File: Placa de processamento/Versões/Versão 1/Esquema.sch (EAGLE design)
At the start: 17 parts, among them IC1 5V, IC2 5V

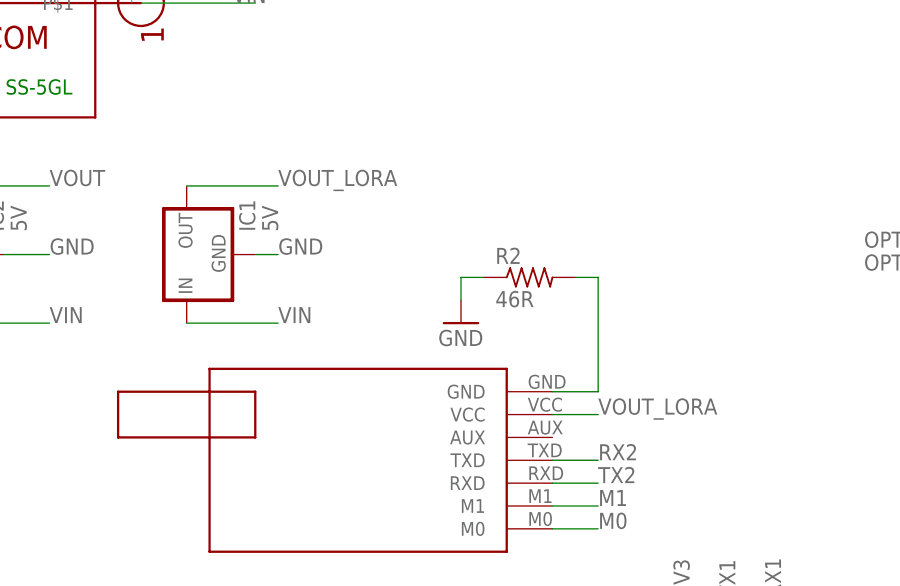
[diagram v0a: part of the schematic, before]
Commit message: uptate boards
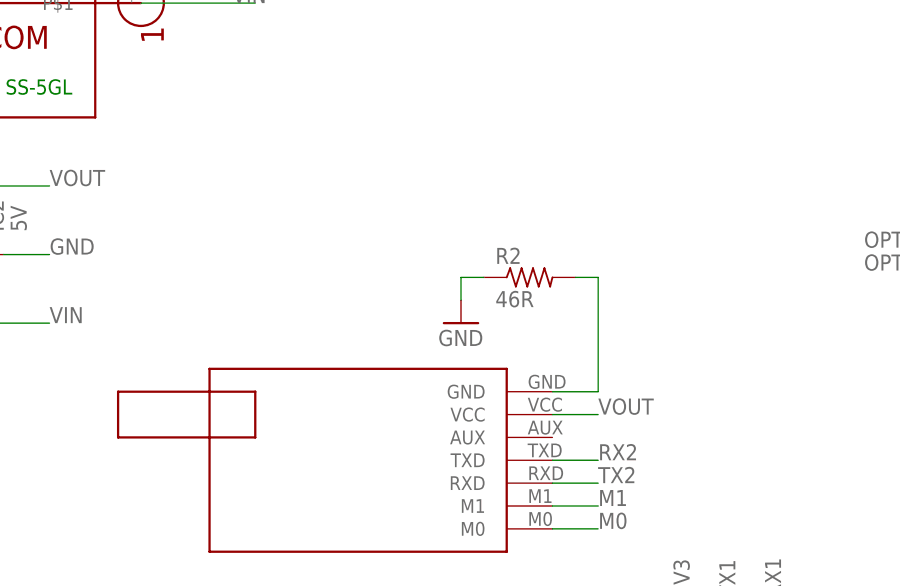
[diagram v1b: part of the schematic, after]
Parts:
- removed IC1: 5V, v-reg:78XXL
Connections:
- removed net VOUT_LORA: IC1.OUT, U$2.VCC
- net GND: no longer IC1.GND
- net VIN: no longer IC1.IN
- net VOUT: now also U$2.VCC
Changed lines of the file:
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@@
 <part name="GND6" library="supply1" library_urn="urn:adsk.eagle:library:371" deviceset="GND" device=""/>
 <part name="SP1" library="buzzer" library_urn="urn:adsk.eagle:library:113" deviceset="AL60P" device="" package3d_urn="urn:adsk.eagle:package:5261/1"/>
-<part name="IC1" library="v-reg" library_urn="urn:adsk.eagle:library:409" deviceset="78XXL" device="" package3d_urn="urn:adsk.eagle:package:30361/1" value="5V"/>
 </parts>
 <sheets>
@@
 <attribute name="VALUE" x="69.215" y="-49.53" size="1.778" layer="96" rot="R90"/>
 </instance>
-<instance part="IC1" gate="A" x="-40.64" y="15.24" smashed="yes" rot="R90">
-<attribute name="NAME" x="-33.02" y="17.78" size="1.778" layer="95" rot="R90"/>
-<attribute name="VALUE" x="-30.48" y="17.78" size="1.778" layer="96" rot="R90"/>
-</instance>
 </instances>
 <busses>
@@
 <label x="-55.88" y="7.62" size="1.778" layer="95"/>
 </segment>
-<segment>
-<pinref part="IC1" gate="A" pin="IN"/>
-<wire x1="-40.64" y1="7.62" x2="-30.48" y2="7.62" width="0.1524" layer="91"/>
-<label x="-30.48" y="7.62" size="1.778" layer="95"/>
-</segment>
 </net>
 <net name="V_BATTERY" class="0">
@@
 <label x="50.292" y="-9.398" size="1.778" layer="95"/>
 </segment>
-<segment>
-<pinref part="IC1" gate="A" pin="GND"/>
-<wire x1="-33.02" y1="15.24" x2="-30.48" y2="15.24" width="0.1524" layer="91"/>
-<label x="-30.48" y="15.24" size="1.778" layer="95"/>
-</segment>
 </net>
 <net name="N$4" class="0">
@@
 <wire x1="-68.58" y1="22.86" x2="-55.88" y2="22.86" width="0.1524" layer="91"/>
 <label x="-55.88" y="22.86" size="1.778" layer="95"/>
+</segment>
+<segment>
+<pinref part="U$2" gate="LORA_E22400T30D" pin="VCC"/>
+<wire x1="5.08" y1="-2.54" x2="0" y2="-2.54" width="0.1524" layer="91"/>
+<label x="5.08" y="-2.54" size="1.778" layer="95"/>
 </segment>
 </net>
@@
 </segment>
 </net>
-<net name="VOUT_LORA" class="0">
-<segment>
-<pinref part="IC1" gate="A" pin="OUT"/>
-<wire x1="-40.64" y1="22.86" x2="-30.48" y2="22.86" width="0.1524" layer="91"/>
-<label x="-30.48" y="22.86" size="1.778" layer="95"/>
-</segment>
-<segment>
-<pinref part="U$2" gate="LORA_E22400T30D" pin="VCC"/>
-<wire x1="5.08" y1="-2.54" x2="0" y2="-2.54" width="0.1524" layer="91"/>
-<label x="5.08" y="-2.54" size="1.778" layer="95"/>
-</segment>
-</net>
